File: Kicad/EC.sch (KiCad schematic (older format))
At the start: 2 parts

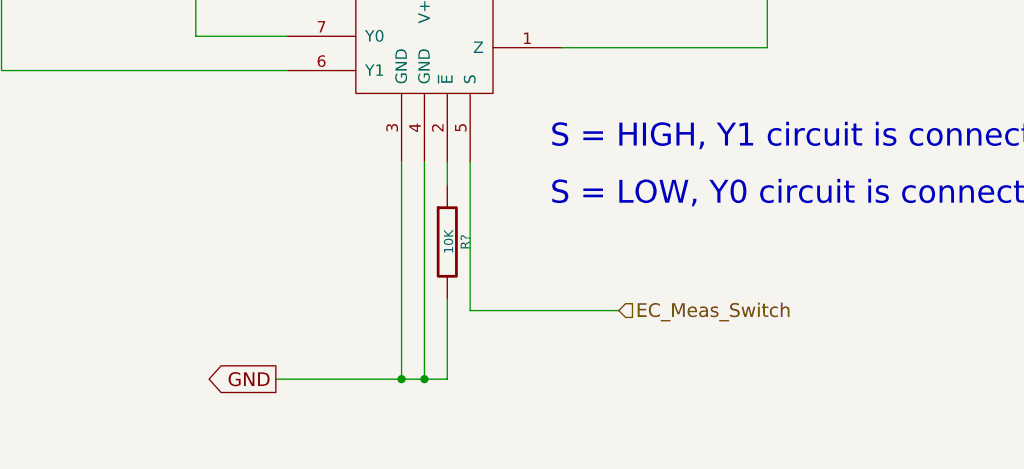
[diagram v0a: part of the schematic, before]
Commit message: check in before modifying Layout with updated design
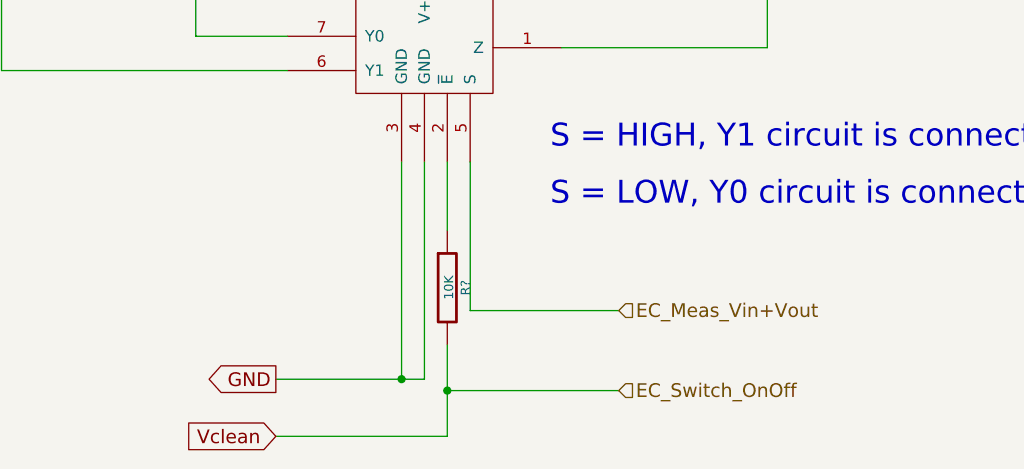
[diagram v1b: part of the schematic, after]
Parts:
- removed R?: 10K, ~, symbol R
- added R?: 10K, ~, symbol R
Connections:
- net Vclean: now also R?.2
- net at U?.2 (~E): now also R?.1
- net EC_Meas_Switch renamed EC_Meas_Vin+Vout
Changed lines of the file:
@@
 Sheet 5 11
 Title ""
-Date "29 jan 2015"
+Date "31 jan 2015"
 Rev ""
 Comp ""
@@
 D9 E2 BF C4 18 F7 0C 4B 5E B4 8D 6F 67 A1 70 71 C5 12 A3 BD DD C9 B3 93 77 93 9B 2B F6 BC 6A 4C
 31 A6 9D A4 5C 5A 6D B5 D5 56 5B 6D B5 D5 02 ED 0F 8F D8 15 DB 22 89 0B B4 00 00 00 00 49 45 4E
-44 AE 42 60 82 A9 $EndBitmap
+44 AE 42 60 82 0B $EndBitmap
 EndData
 $EndBitmap
@@
 12 D7 1E 39 D3 97 8B E9 CC 09 7E A4 21 84 7B DE 75 BE 6C 10 1D B1 C0 C8 E6 44 20 98 58 88 D3 4B
 BF A4 FE AC E7 27 87 F5 F3 E7 B2 6E 04 7A D3 5E FF 1F 0B 1A 44 E2 12 6D EC E1 00 00 00 00 49 45
-4E 44 AE 42 60 82 68 $EndBitmap
+4E 44 AE 42 60 82 69 $EndBitmap
 EndData
 $EndBitmap
@@
 GND
 Wire Wire Line
-	5000 6800 5750 6800
-Wire Wire Line
-	5650 5850 5650 6800
-$Comp
-L R R?
-U 1 1 54C7AE26
-P 5750 6200
-F 0 "R?" V 5830 6200 40  0000 C CNN
-F 1 "10K" V 5757 6201 40  0000 C CNN
-F 2 "~" V 5680 6200 30  0000 C CNN
-F 3 "~" H 5750 6200 30  0000 C CNN
-	1    5750 6200
-	1    0    0    -1
-$EndComp
+	5650 6800 5650 5850
 Wire Wire Line
 	5550 6800 5550 5850
-Connection ~ 5550 6800
-Wire Wire Line
-	5750 5950 5750 5850
-Wire Wire Line
-	5750 6800 5750 6450
-Connection ~ 5650 6800
+Wire Wire Line
+	5750 5850 5750 6150
 Text HLabel 6500 6500 2    60   Input ~ 0
-EC_Meas_Switch
+EC_Meas_Vin+Vout
 Wire Wire Line
 	5850 5850 5850 6500
@@
 Text Notes 6200 6050 0    100  ~ 0
 S = LOW, Y0 circuit is connected (measure EC_DCv)
+$Comp
+L R R?
+U 1 1 54CBB29D
+P 5750 6400
+F 0 "R?" V 5830 6400 40  0000 C CNN
+F 1 "10K" V 5757 6401 40  0000 C CNN
+F 2 "~" V 5680 6400 30  0000 C CNN
+F 3 "~" H 5750 6400 30  0000 C CNN
+	1    5750 6400
+	1    0    0    -1
+$EndComp
+Wire Wire Line
+	5000 6800 5650 6800
+Connection ~ 5550 6800
+Wire Wire Line
+	5750 6650 5750 7050
+Wire Wire Line
+	5750 7050 5000 7050
+Text GLabel 5000 7050 0    60   Input ~ 0
+Vclean
+Text HLabel 6500 6850 2    60   Input ~ 0
+EC_Switch_OnOff
+Wire Wire Line
+	6500 6850 5750 6850
+Connection ~ 5750 6850
 $EndSCHEMATC
